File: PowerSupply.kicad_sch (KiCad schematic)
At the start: 23 parts, among them J6 PWR, J7 uC PTT, K3 G5V-2, Q3 2N3904, U7 LM7805, U8 LM7808

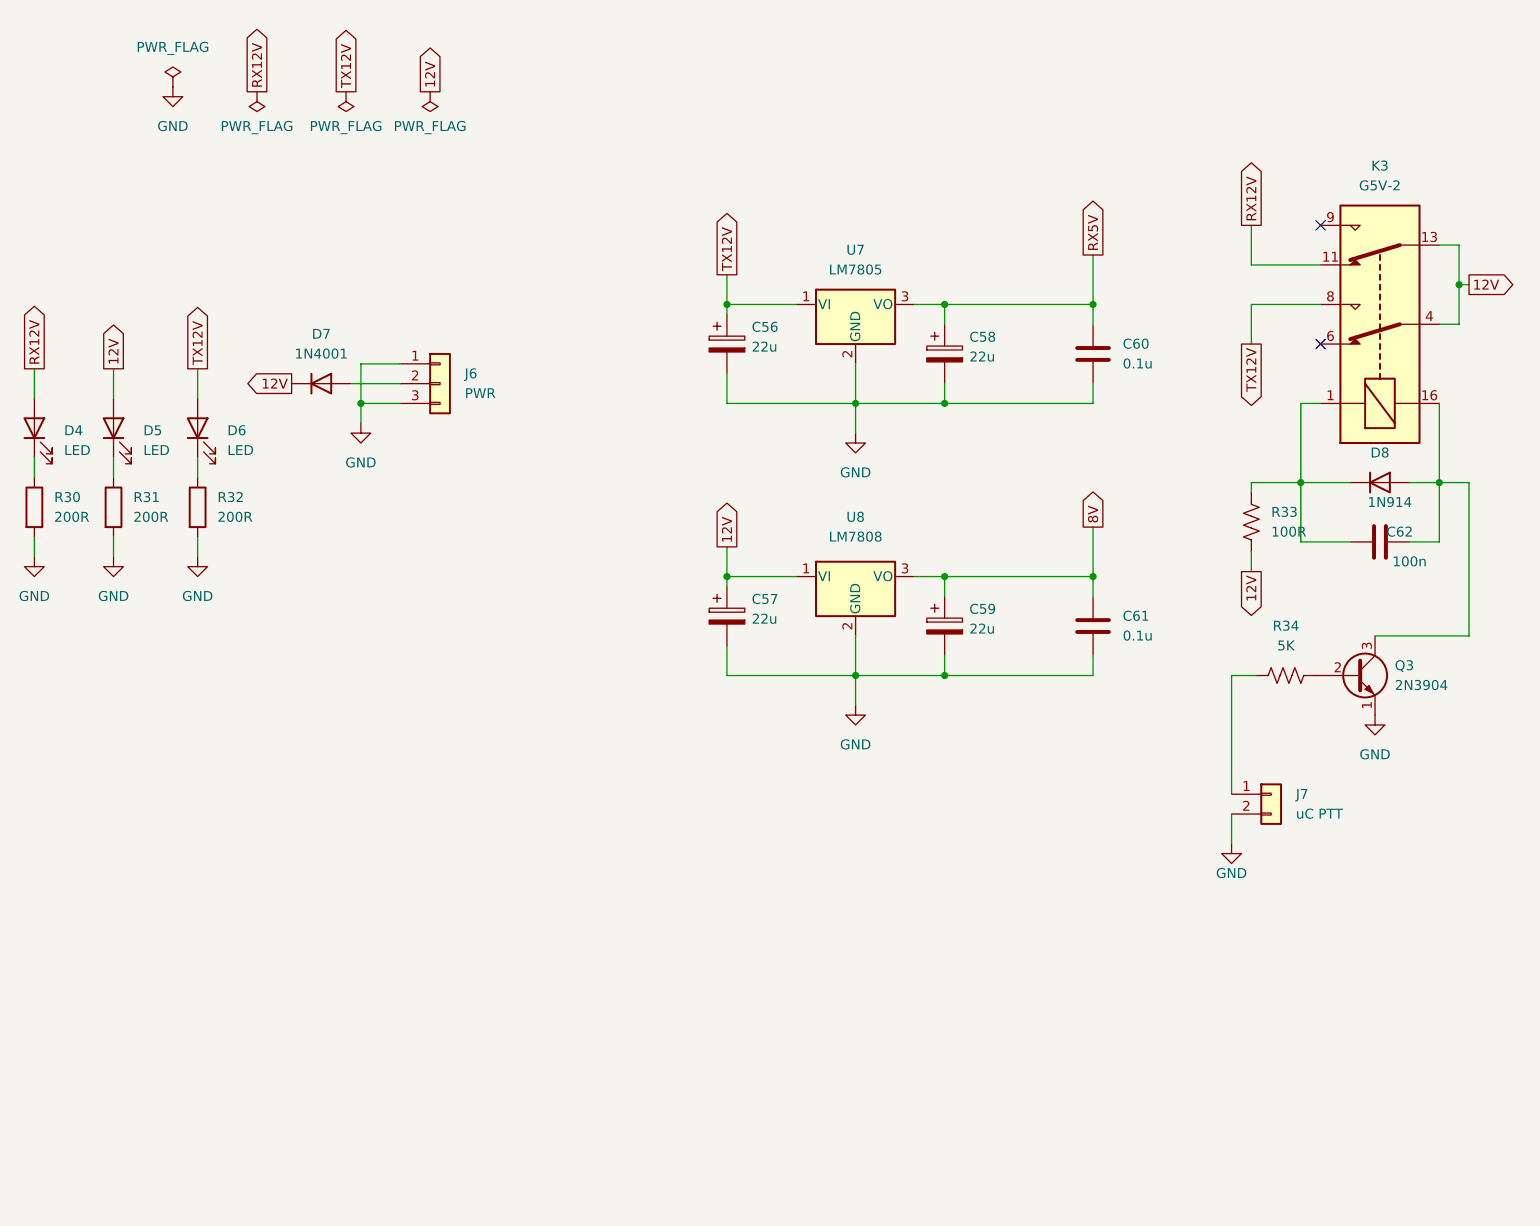
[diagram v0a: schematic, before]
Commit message: Update
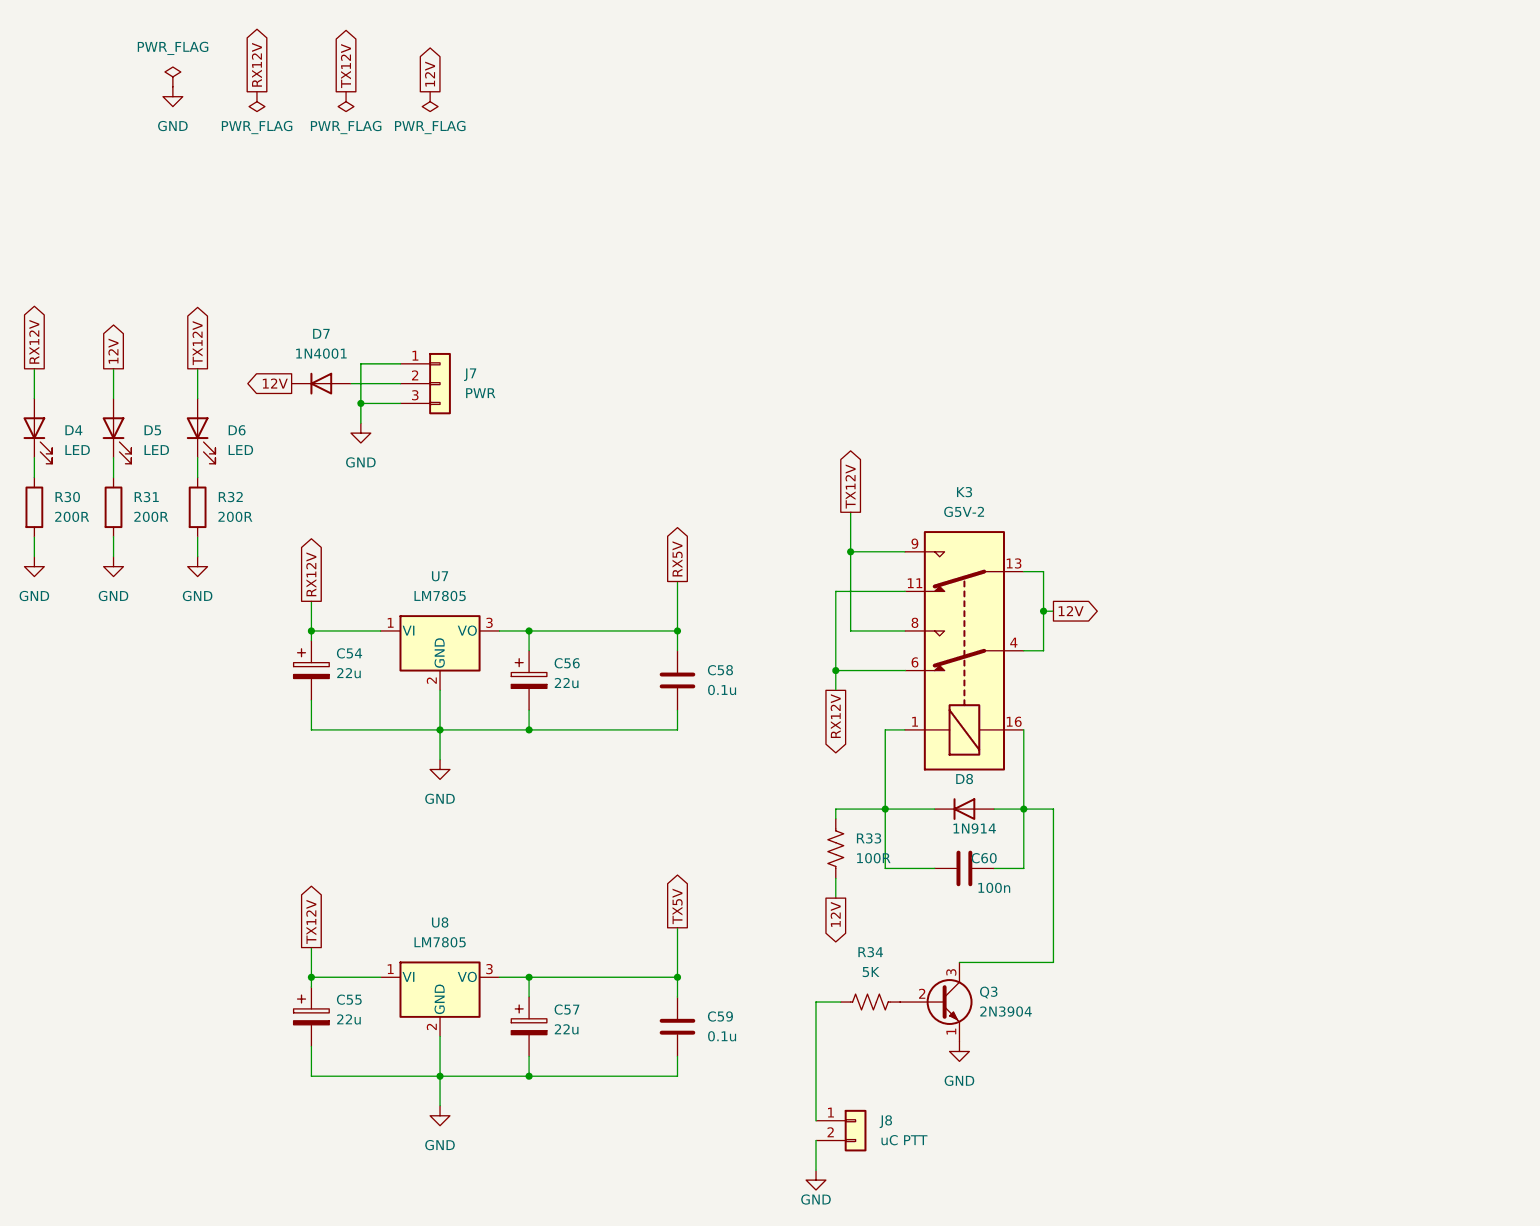
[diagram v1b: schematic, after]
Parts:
- removed C59: 22u, Capacitor_THT:CP_Radial_D8.0mm_P2.50mm, symbol Device:C_Polarized
- removed C61: 0.1u, Capacitor_THT:C_Disc_D3.0mm_W1.6mm_P2.50mm, symbol Device:C
- removed U8: LM7808, Package_TO_SOT_THT:TO-220-3_Vertical, symbol Regulator_Linear:LM7808_TO220
- added C55: 22u, Capacitor_THT:CP_Radial_D8.0mm_P2.50mm, symbol Device:C_Polarized
- added C59: 0.1u, Capacitor_THT:C_Disc_D3.0mm_W1.6mm_P2.50mm, symbol Device:C
- added U8: LM7805, Package_TO_SOT_THT:TO-220-3_Vertical, symbol Regulator_Linear:LM7805_TO220
- renumbered C56 to C54, C58 to C56, C60 to C58, C62 to C60, J6 to J7, J7 to J8
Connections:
- net 12V: no longer C57.1
- net GND: now also C55.2, C59.2, U8.2 (GND)
- net RX12V: now also C54.1, K3.6, U7.1 (VI)
- net TX12V: now also K3.9, C55.1, U8.1 (VI); no longer C54.1, U7.1 (VI)
- new net TX5V: C57.1, C59.1, U8.3 (VO)
- no-connect marks 2 -> 0
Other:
- moved on the sheet: C54, C56, C58, C60, D8, J8, K3, Q3, R33, R34, U7
